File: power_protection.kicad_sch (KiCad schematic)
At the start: 10 parts, among them Q901 AO3401A, Q902 AO3401A

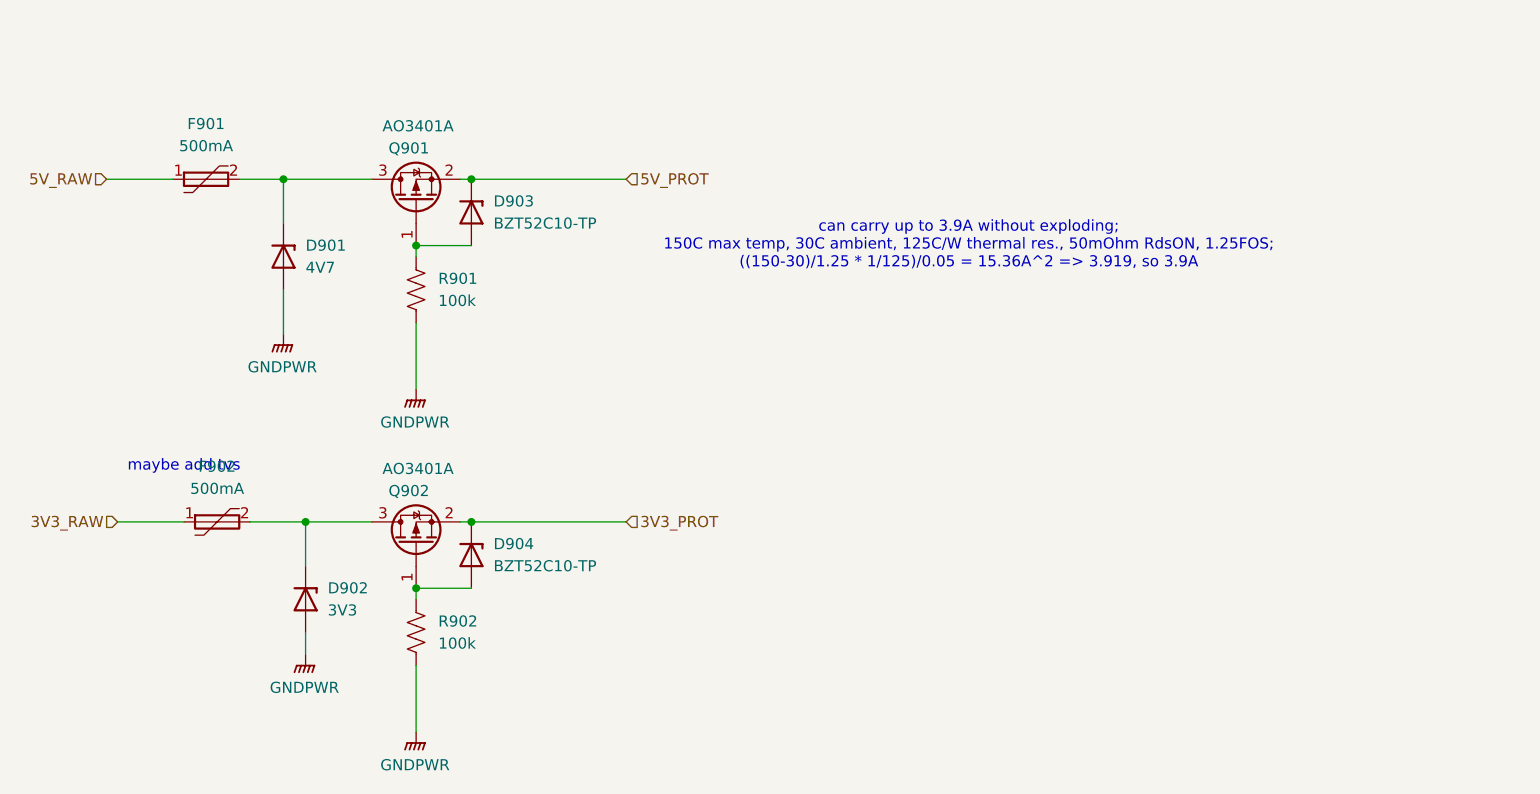
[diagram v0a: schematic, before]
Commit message: fixed like a bunch of things, power and new xcvr and lights and other goodies, also started layout
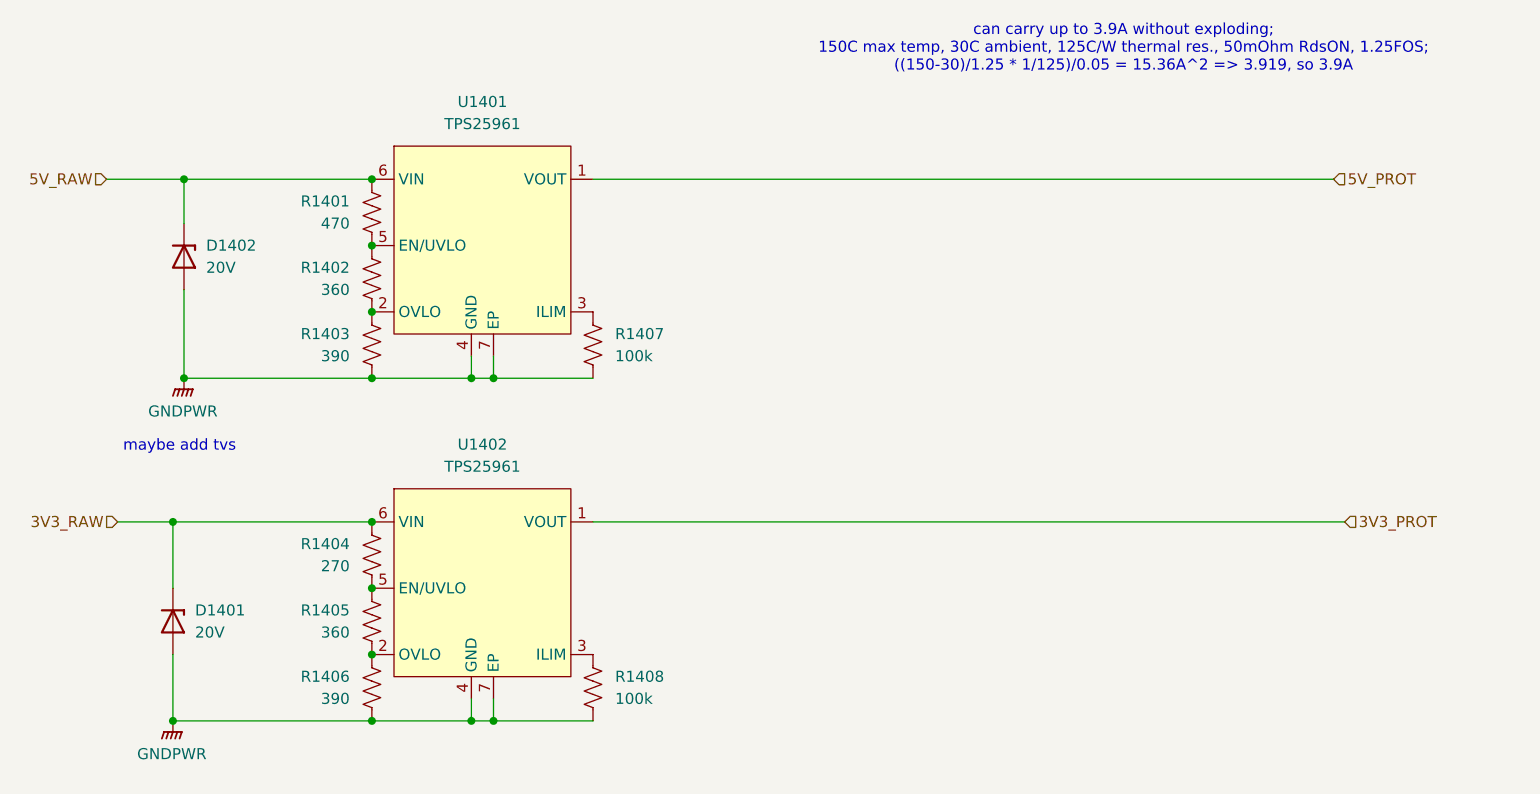
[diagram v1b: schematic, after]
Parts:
- removed D901: 4V7, Diode_SMD:D_SMB, symbol bfr_diodes:1SMB5917BT3G
- removed D902: 3V3, Diode_SMD:D_SMB, symbol bfr_diodes:1SMB5913BT3G
- removed D903, D904: BZT52C10-TP, Diode_SMD:D_SOD-123, symbol bfr_diodes:BZT52C10
- removed F901, F902: 500mA, Fuse:Fuse_1812_4532Metric, symbol bfr_utilities:0ZCG0050AF2C
- removed Q901, Q902: AO3401A, Package_TO_SOT_SMD:SOT-23-3, symbol Device:Q_PMOS_GSD
- removed R901, R902: 100k, Resistor_SMD:R_0603_1608Metric_Pad0.98x0.95mm_HandSolder, symbol bfr_resistors:RMCF0603FT100K
- added D1401, D1402: 20V, Diode_SMD:D_SMB, symbol bfr_diodes:1SMB5932BT3G
- added R1401: 470, Resistor_SMD:R_0402_1005Metric_Pad0.72x0.64mm_HandSolder, symbol bfr_resistors:RMCF0402FT470R
- added R1402, R1405: 360, Resistor_SMD:R_0603_1608Metric_Pad0.98x0.95mm_HandSolder, symbol bfr_resistors:RMCF0603FT360R
- added R1403, R1406: 390, Resistor_SMD:R_0603_1608Metric_Pad0.98x0.95mm_HandSolder, symbol bfr_resistors:RMCF0603FT390R
- added R1404: 270, Resistor_SMD:R_0603_1608Metric_Pad0.98x0.95mm_HandSolder, symbol bfr_resistors:RMCF0603FT270R
- added R1407, R1408: 100k, Resistor_SMD:R_0402_1005Metric_Pad0.72x0.64mm_HandSolder, symbol bfr_resistors:RMCF0402FT100K
- added U1401, U1402: TPS25961, Package_SON:WSON-6-1EP_2x2mm_P0.65mm_EP1x1.6mm, symbol bfr_power_ics:TPS25961
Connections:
- net 3V3_PROT: now also U1402.1 (VOUT)
- net 3V3_RAW: now also D1401.1 (K), R1404.2, U1402.6 (VIN)
- net 5V_PROT: now also U1401.1 (VOUT)
- net 5V_RAW: now also D1402.1 (K), R1401.2, U1401.6 (VIN)
- net GNDPWR: now also D1401.2 (A), D1402.2 (A), R1403.1, R1406.1, R1407.1, R1408.1, U1401.4 (GND), U1401.7 (EP), U1402.4 (GND), U1402.7 (EP)
- new net: R1401.1, R1402.2, U1401.5 (EN/UVLO)
- new net: R1405.1, R1406.2, U1402.2 (OVLO)
- new net: R1408.2, U1402.3 (ILIM)
- new net: R1404.1, R1405.2, U1402.5 (EN/UVLO)
- new net: R1402.1, R1403.2, U1401.2 (OVLO)
- new net: R1407.2, U1401.3 (ILIM)
